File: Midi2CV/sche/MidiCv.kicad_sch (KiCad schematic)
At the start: 9 parts, among them U1 STM32F103C8T6_BD, U2 6N138

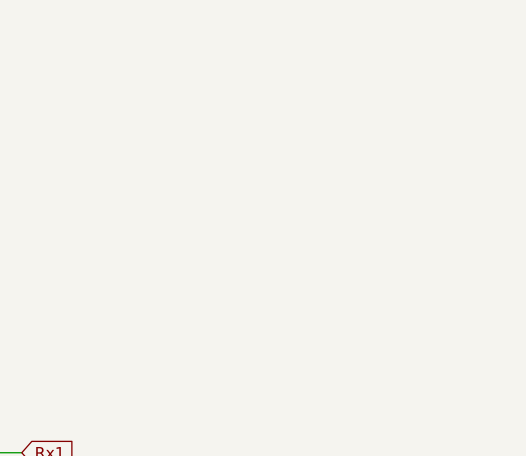
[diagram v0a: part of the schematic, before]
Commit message: re - revert
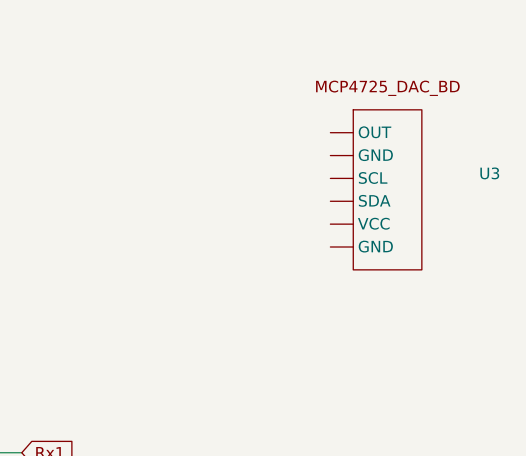
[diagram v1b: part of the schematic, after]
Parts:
- added U3: ~, symbol RetroElec:MCP4725_DAC_BD
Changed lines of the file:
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@@
+    )
+  )
+  (symbol (lib_id "RetroElec:MCP4725_DAC_BD") (at 195.58 54.61 0) (unit 1)
+    (in_bom yes) (on_board yes) (dnp no) (fields_autoplaced)
+    (property "Reference" "U3" (at 205.74 52.8292 0)
+      (effects (font (size 1.27 1.27)) (justify left))
+    )
+    (property "Value" "~" (at 194.31 52.07 0)
+      (effects (font (size 1.27 1.27)))
+    )
+    (property "Footprint" "" (at 194.31 52.07 0)
+      (effects (font (size 1.27 1.27)) hide)
+    )
+    (property "Datasheet" "" (at 194.31 52.07 0)
+      (effects (font (size 1.27 1.27)) hide)
+    )
+    (pin "")
+    (pin "")
+    (pin "")
+    (pin "")
+    (pin "")
+    (pin "")
+    (instances
+      (project "MidiCv"
+        (path "/0e81e7e9-28eb-4e3c-9e5d-03b0357b6be8"
+          (reference "U3") (unit 1)
+        )
+      )
     )
   )
